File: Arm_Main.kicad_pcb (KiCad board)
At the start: 2 copper layers, 100 x 80 mm, 58 parts, among them IC1 TLP559_F_, IC2 TLP559_F_, J1 Conn_01x02_Pin, J2 Conn_01x03_Socket, J3 Conn_01x03_Pin, J4 Conn_01x03_Pin, J5 Conn_01x03_Pin, SW1 SW_SPST, SW2 SW_SPST, SW3 SW_SPST, U1 ADuM121N, U2 TLP2531, U3 RASPBERRY_PI_ZERO_2_W, U4 LM350_TO220

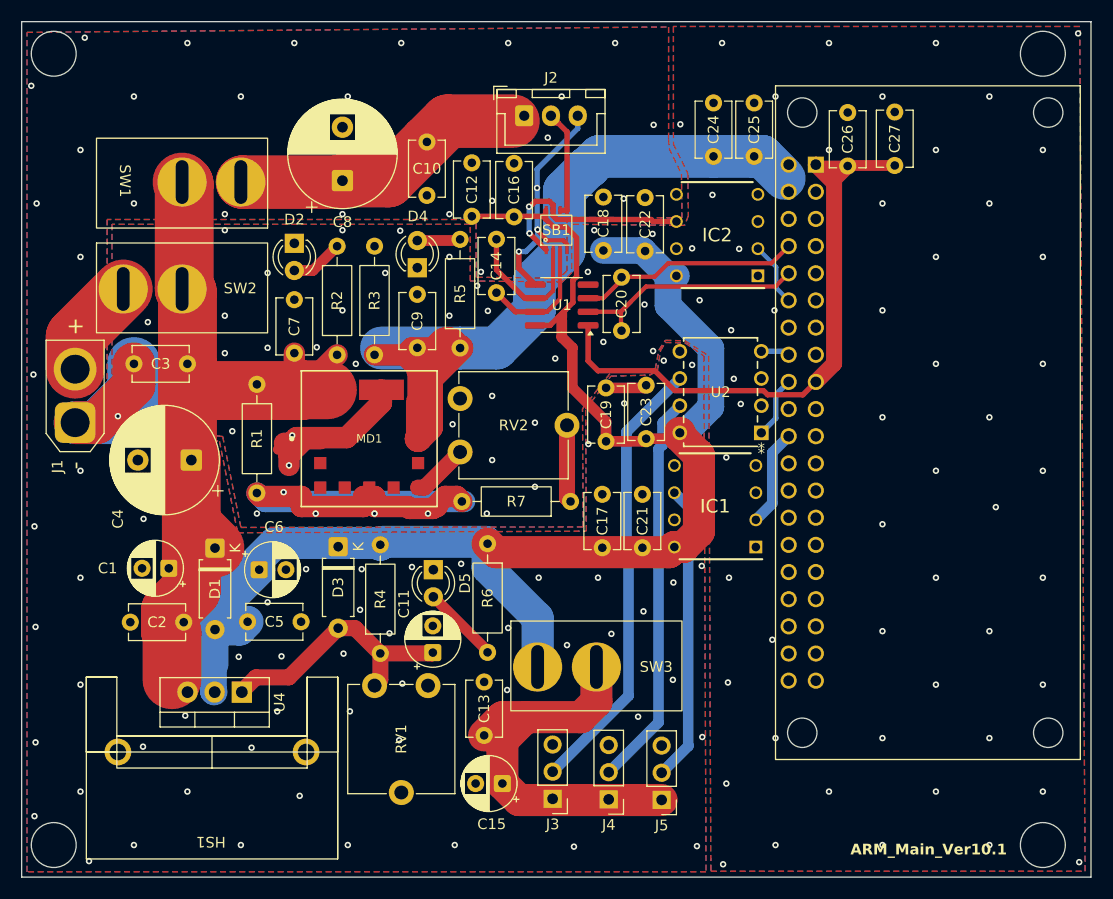
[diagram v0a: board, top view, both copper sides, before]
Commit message: ver10.1
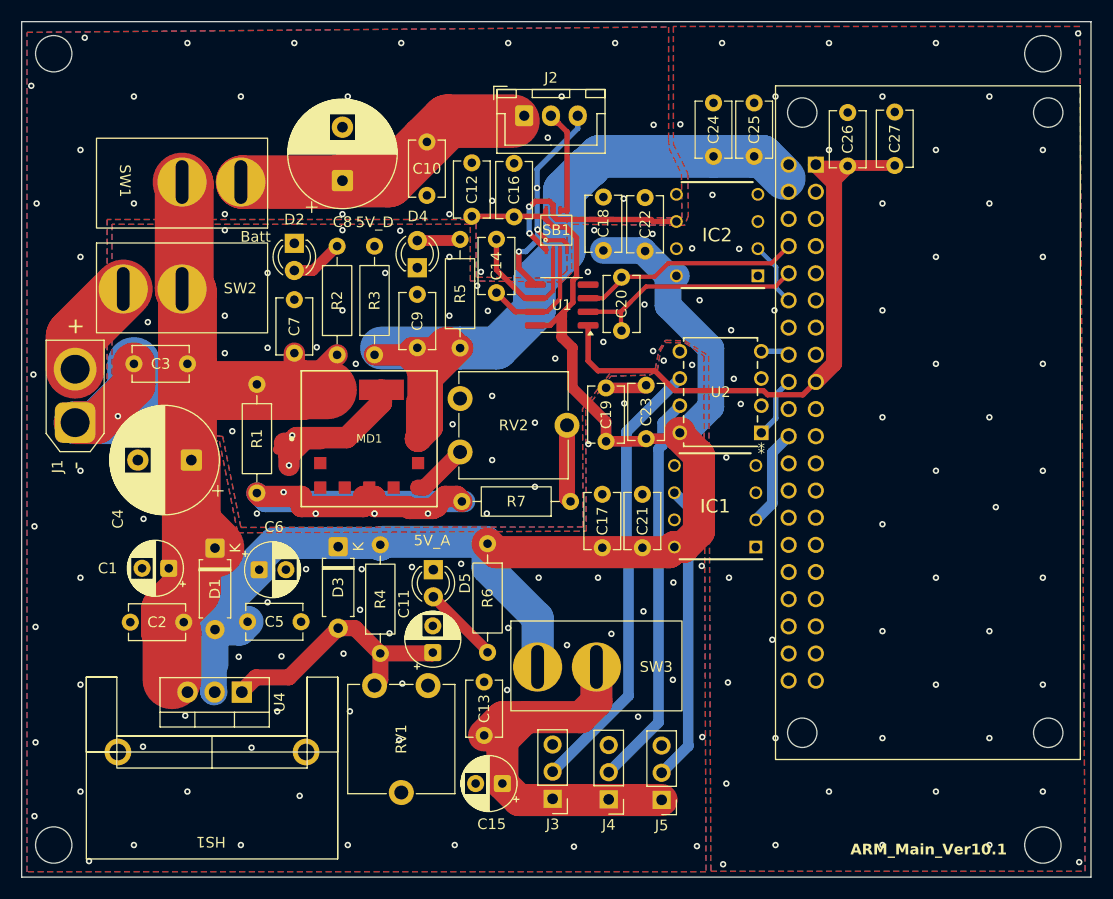
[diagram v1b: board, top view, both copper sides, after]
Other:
- outline, holes or cut-outs redrawn
- board text added: "5V_A"
- board text added: "5V_D"
- board text added: "Batt"
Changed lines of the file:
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@@
 	(gr_circle
 		(center 102.5 130)
-		(end 104.6 130)
+		(end 104.2 130)
 		(stroke
 			(width 0.05)
@@
 	(gr_circle
 		(center 195 56)
-		(end 197.1 56)
+		(end 196.7 56)
 		(stroke
 			(width 0.05)
@@
 	(gr_circle
 		(center 102.5 56)
-		(end 104.6 56)
+		(end 104.2 56)
 		(stroke
 			(width 0.05)
@@
 	(gr_circle
 		(center 195 130)
-		(end 197.1 130)
+		(end 196.7 130)
 		(stroke
 			(width 0.05)
@@
 		(fill no)
 		(layer "Edge.Cuts")
+	)
+	(gr_text "Batt"
+		(at 119.95 73.7 0)
+		(layer "F.SilkS")
+		(effects
+			(font
+				(size 1 1)
+				(thickness 0.1)
+			)
+			(justify left bottom)
+		)
+	)
+	(gr_text "5V_D"
+		(at 130.74 72.34 0)
+		(layer "F.SilkS")
+		(effects
+			(font
+				(size 1 1)
+				(thickness 0.1)
+			)
+			(justify left bottom)
+		)
 	)
 	(gr_text "ARM_Main_Ver10.1"
@@
 			)
 			(justify left bottom)
+		)
+	)
+	(gr_text "5V_A"
+		(at 136.16 102.1 0)
+		(layer "F.SilkS")
+		(effects
+			(font
+				(size 1 1)
+				(thickness 0.1)
+			)
+			(justify left bottom)
